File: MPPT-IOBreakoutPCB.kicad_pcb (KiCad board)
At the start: 2 copper layers, 4 parts, among them J1 Conn_01x06, J2 Conn_01x06, J3 Conn_01x06

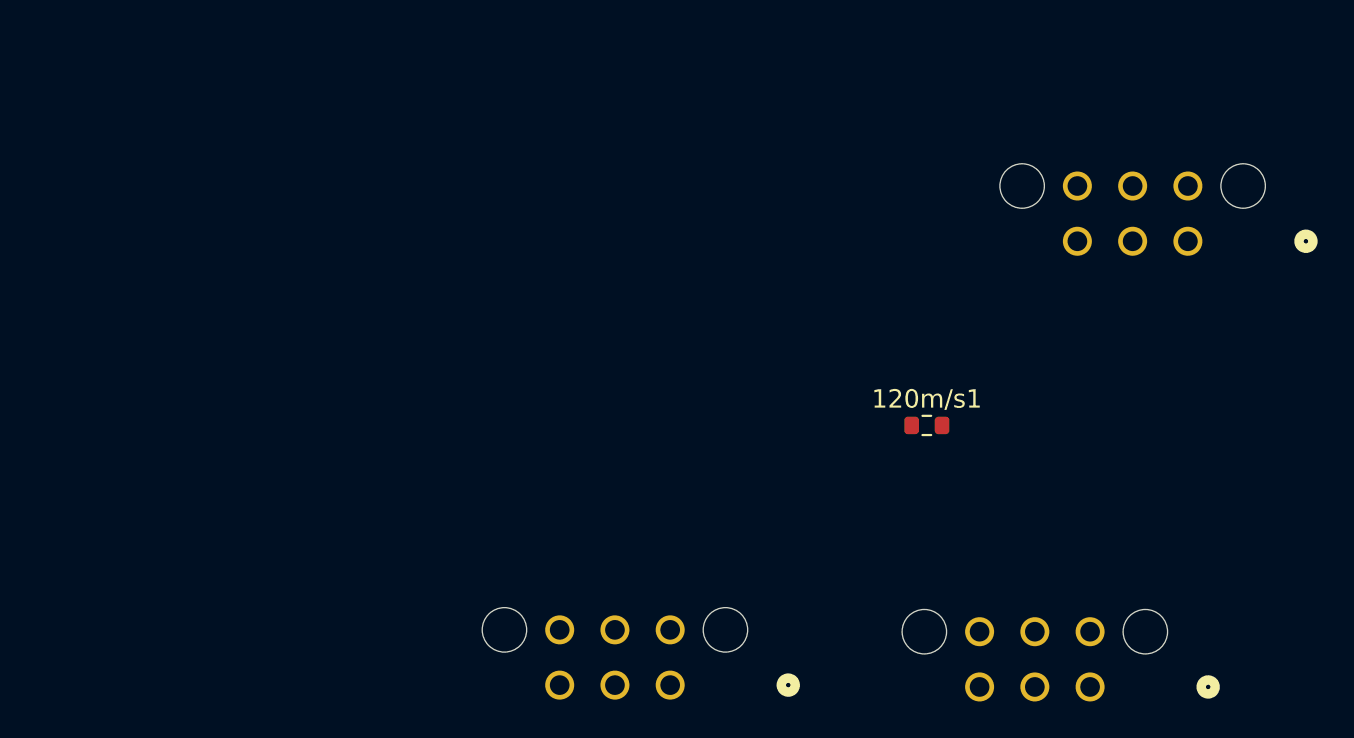
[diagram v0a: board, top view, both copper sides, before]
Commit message: layout maybe done
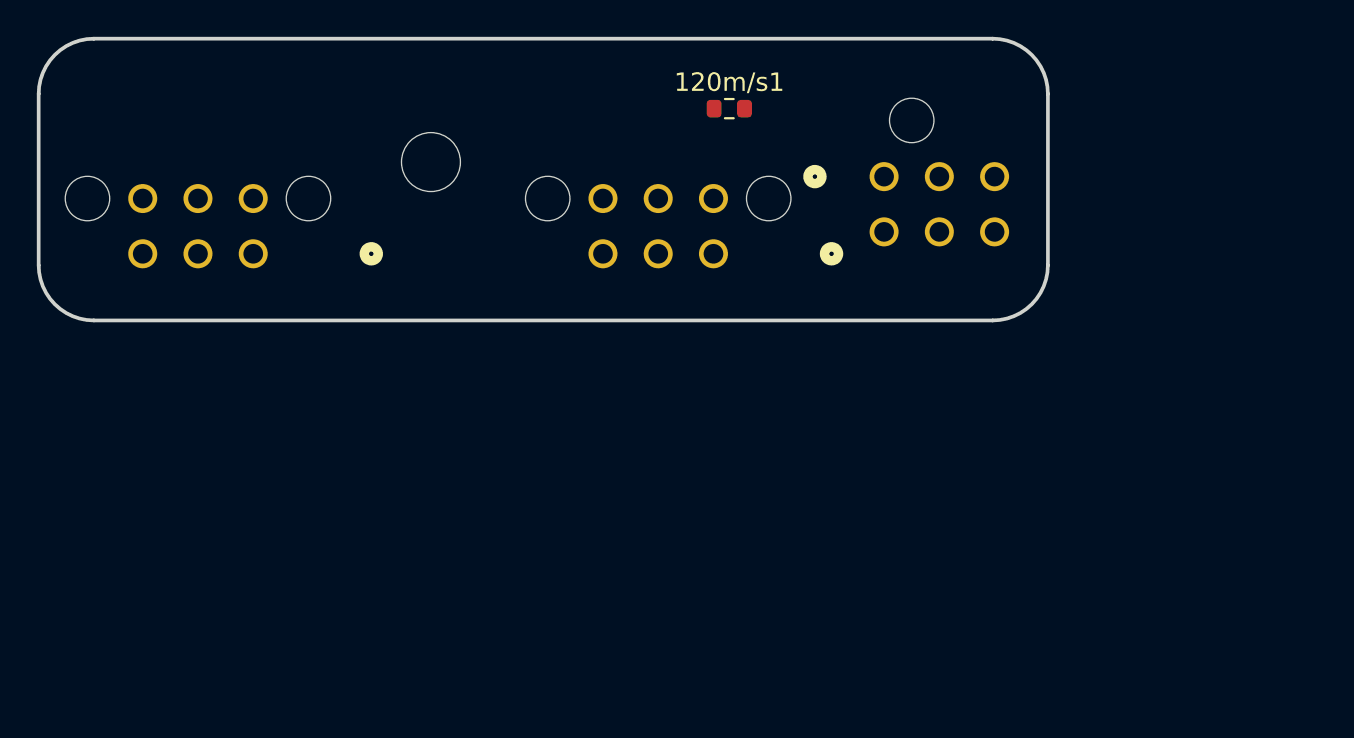
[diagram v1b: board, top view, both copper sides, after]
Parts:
- added REF**: MountingHole_3.2mm_M3, MountingHole:MountingHole_3.2mm_M3, F.Cu at (123.5, 87.7)
- J3: footprint UTSVT_Connectors:Molex_Microfit3.0_02x03_6-Pin-Vertical-PCB-Receptacle_447690601 -> footprints:CONN_SD-44764-001_06_MOL
- moved J2 32.6 mm to (113.8, 92.7)
- moved J1 31.2 mm to (138.8, 92.7)
- moved 120m/s1 20.3 mm to (139.7, 84.8)
- moved J3 16.9 mm to (148.1, 88.5), turned to 0 degrees
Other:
- board outline added: 54.8 x 15.3 mm
- board text added: "For Instructional Use Only."
- board text added: "SOLIDWORKS Educational Product."
